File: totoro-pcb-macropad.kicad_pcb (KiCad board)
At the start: 2 copper layers, 57.2 x 79.2 mm, 38 parts

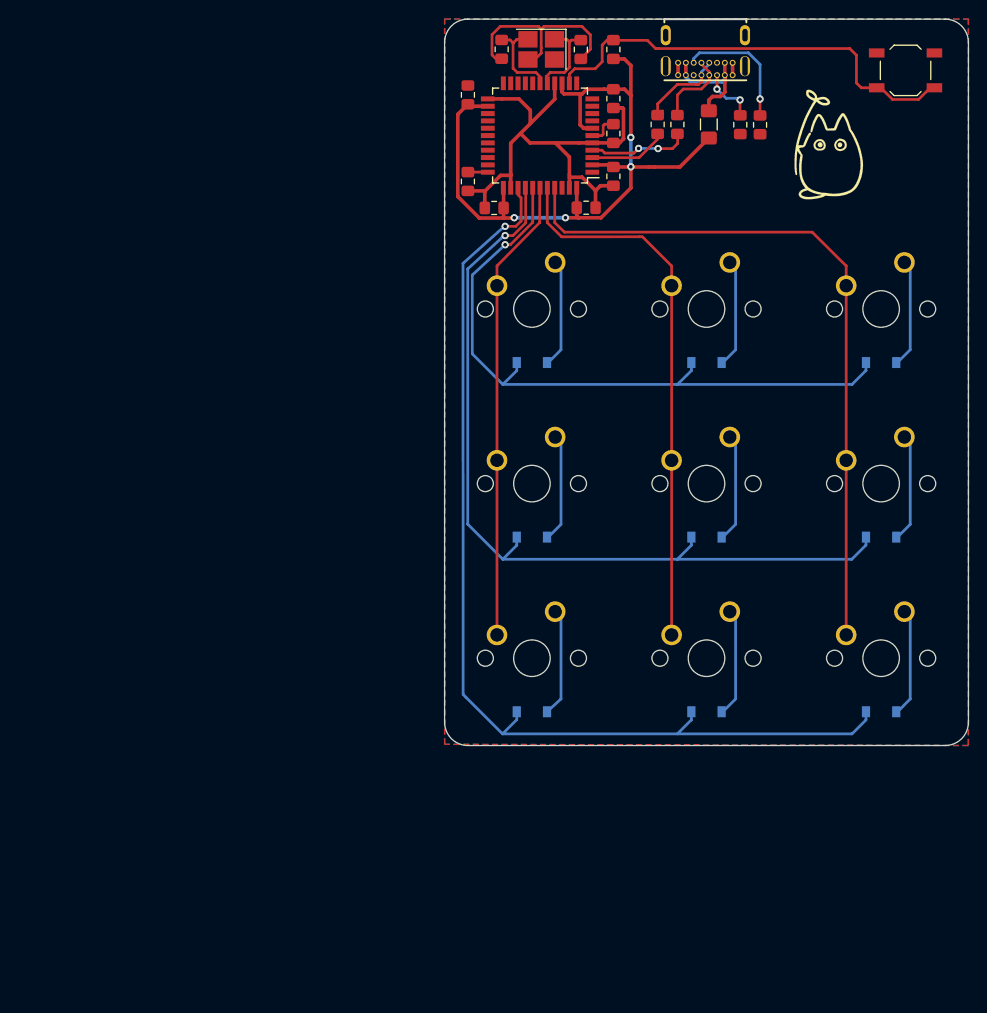
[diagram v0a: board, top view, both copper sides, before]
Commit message: Probably fix crystal footprint, but i dont remember
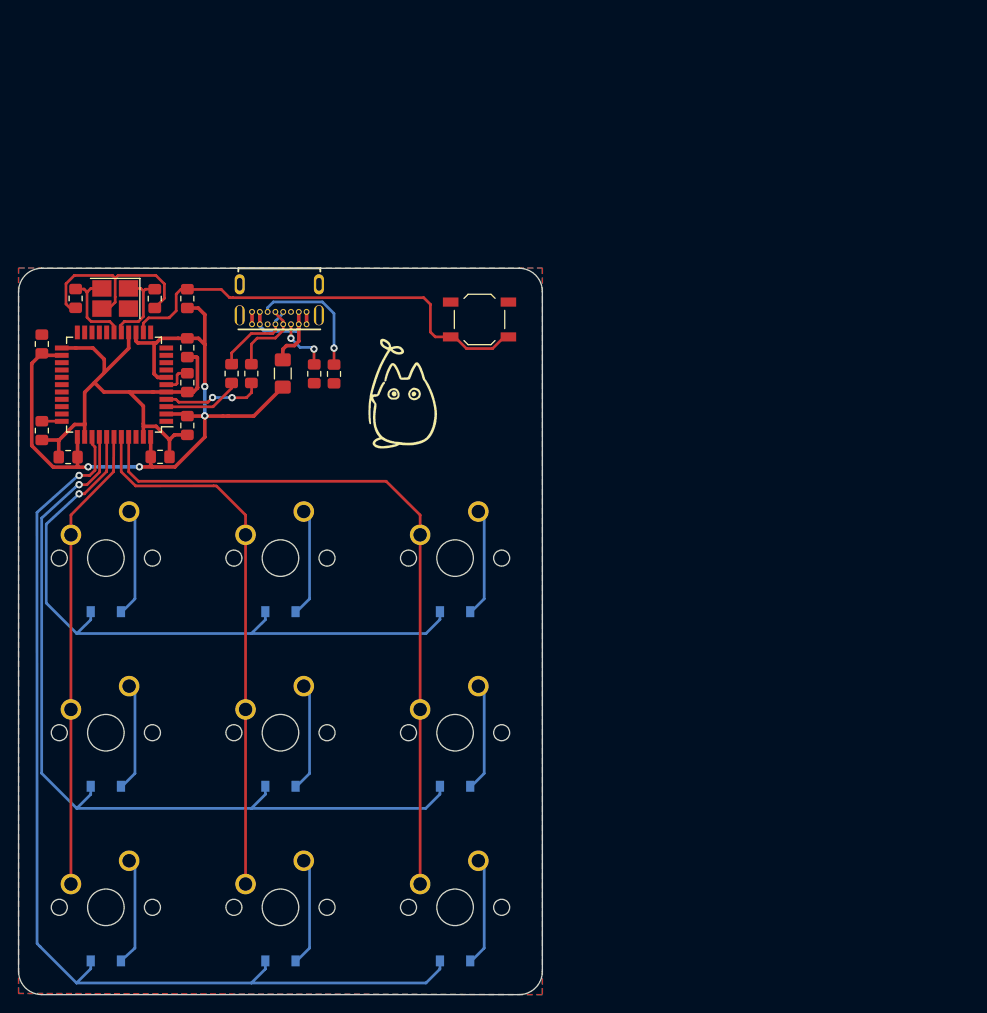
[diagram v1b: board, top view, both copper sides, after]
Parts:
- moved   53.8 mm to (124.8, 59.2)
- moved   53.8 mm to (147.4, 67.4)
- moved   53.8 mm to (137.0, 59.2)
- moved   53.8 mm to (147.1, 58.0)
- moved   53.8 mm to (166.2, 131.4)
- moved   53.8 mm to (147.2, 131.4)
- moved   53.8 mm to (128.1, 131.4)
- moved   53.8 mm to (166.2, 112.4)
- moved   53.8 mm to (147.2, 112.4)
- moved   53.8 mm to (128.1, 112.4)
- moved   53.8 mm to (166.2, 93.3)
- moved   53.8 mm to (147.2, 93.3)
- moved   53.8 mm to (129.2, 59.2)
- moved   53.8 mm to (128.1, 93.3)
- moved   53.8 mm to (137.0, 68.4)
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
